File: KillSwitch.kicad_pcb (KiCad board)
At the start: 2 copper layers, 64 x 31 mm, 28 parts, among them J0 Screw_Terminal_1x04, J3 CONN_01X02, Q0 IRF1324PBF, Q1 IRF1324PBF, Q2 IRF1324PBF, Q3 IRF1324PBF, U0 NC7SZ08, U1 TPS62175, U2 4013

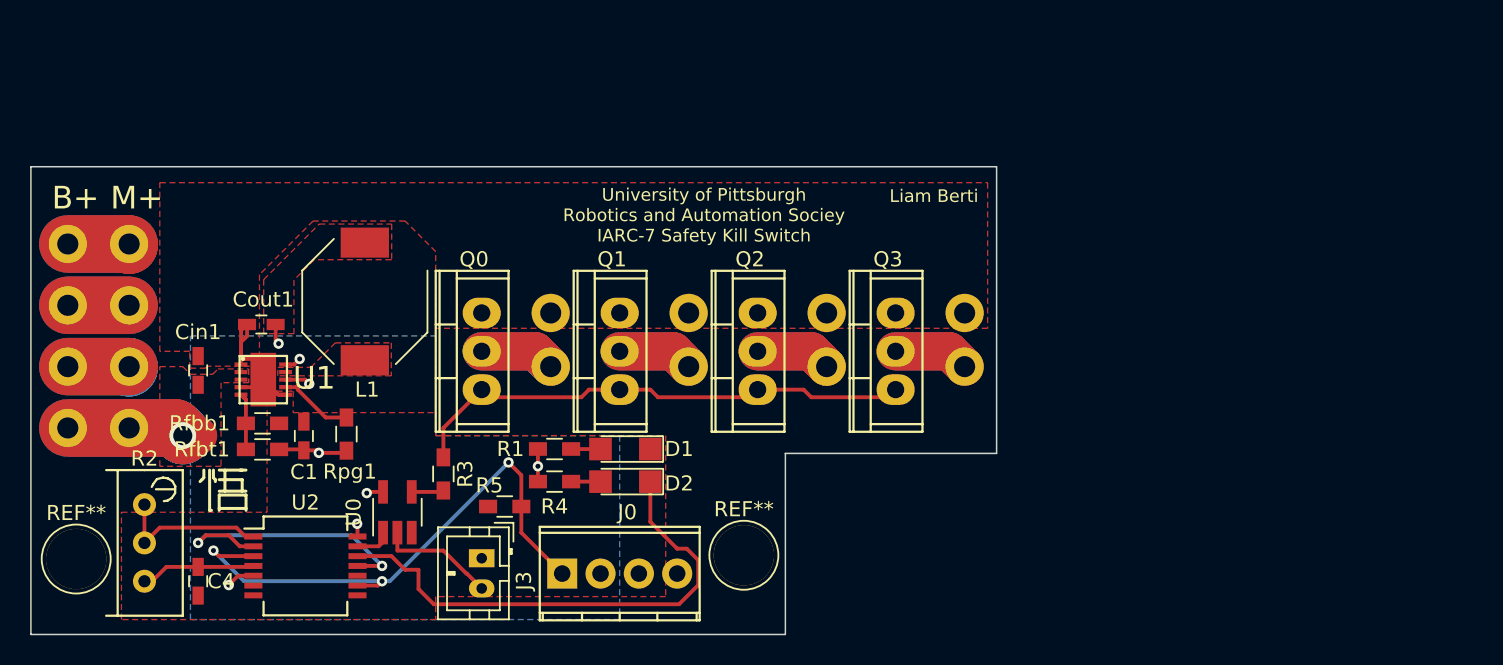
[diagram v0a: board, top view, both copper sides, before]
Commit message: new switch
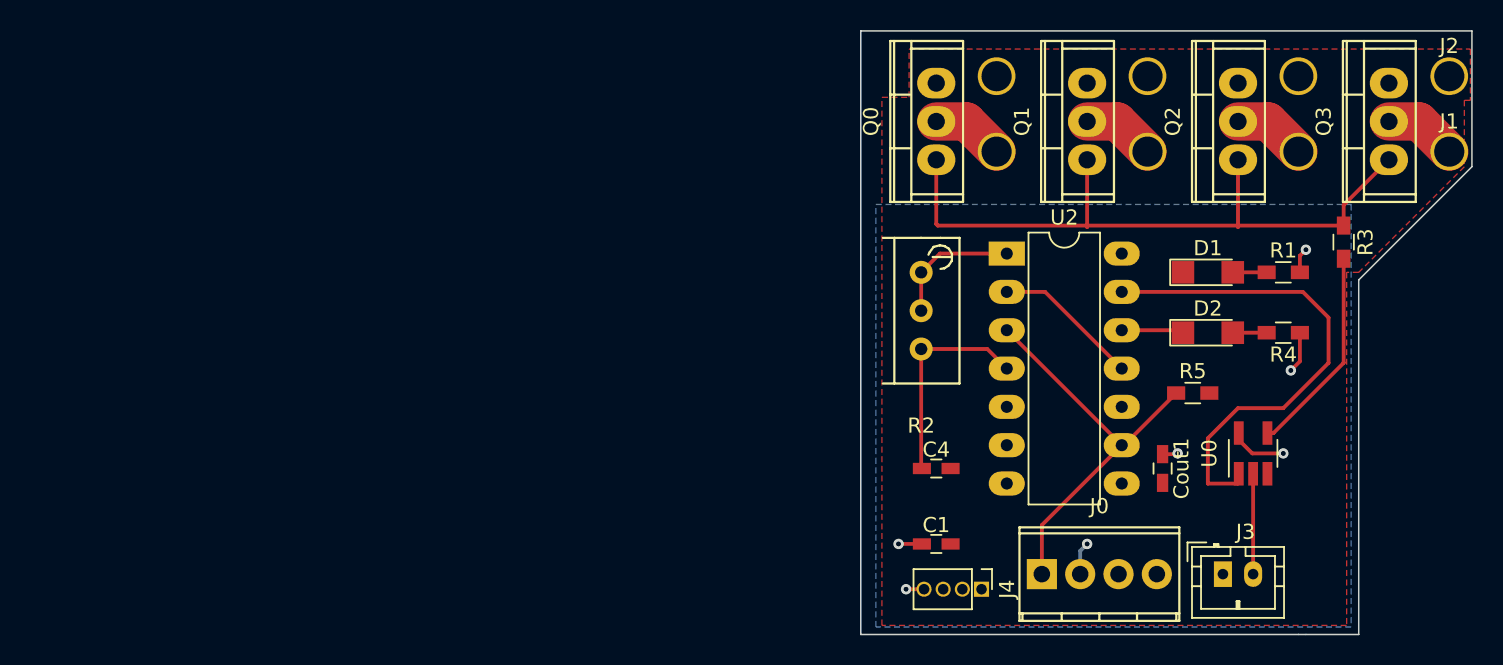
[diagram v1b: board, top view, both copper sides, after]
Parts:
- removed ? (x2): CONN_01X08, Wire_Pads:barrel_connector
- removed Cin1: 2.2uF, Capacitors_SMD:C_0603_HandSoldering
- removed L1: 10uH, 0.036Ohm, Inductors:Inductor_Bourns-SRU8043
- removed REF** (x2): 1pin, UserParts:4mmhole
- removed Rfbb1: 383k, Resistors_SMD:R_0603_HandSoldering
- removed Rfbt1: 2Meg, Resistors_SMD:R_0603_HandSoldering
- removed Rpg1: 100k, Resistors_SMD:R_0603_HandSoldering
- removed U1: TPS62175, Housings_SON:SON-10
- added J1: CONN_01X04, Wire_Pads:barrel_connector, F.Cu at (189.0, 56.0)
- added J2: CONN_01X04, Wire_Pads:barrel_connector, F.Cu at (218.0, 51.0)
- added J4: CONN_01X04, Socket_Strips:Socket_Strip_Straight_1x04_Pitch1.27mm, F.Cu at (184.0, 94.0)
- U2: footprint Housings_SSOP:SSOP-14_5.3x6.2mm_Pitch0.65mm -> Housings_DIP:DIP-14_W7.62mm_LongPads
- moved R3 61.6 mm to (208.0, 71.0)
- moved Cout1 60.5 mm to (196.0, 86.0), turned to 270 degrees
- moved U0 56.8 mm to (202.0, 85.0)
- moved R2 53.7 mm to (180.0, 73.0)
- moved U2 50.9 mm to (185.7, 71.8)
- moved R1 49.7 mm to (204.0, 73.0), turned to 0 degrees
- moved C4 49.5 mm to (181.0, 86.0), turned to 0 degrees
- moved R4 49.3 mm to (204.0, 77.0), turned to 180 degrees
- moved J3 49.1 mm to (200.0, 93.0), turned to 0 degrees
- moved R5 46.2 mm to (198.0, 81.0), turned to 0 degrees
- moved C1 42.5 mm to (181.0, 91.0), turned to 0 degrees
- moved D1 40.3 mm to (199.0, 73.0), turned to 0 degrees
- moved D2 39.8 mm to (199.0, 77.0), turned to 0 degrees
- moved Q3 36.1 mm to (211.0, 63.0)
- moved Q2 35.3 mm to (201.0, 63.0)
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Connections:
- J0 pad 4: Net-(J0-Pad4) -> (no net)
- U2 pad 7: VSS -> Earth
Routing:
- net /AND1: track 2.41 -> 33.1 mm
- net Net-(D2-Pad1): track 33.7 -> 4.36 mm
- net /VbattPos: track 18.1 -> 0.00 mm, vias 2 -> 0
- net Earth: track 13.6 -> 0.00 mm
- net Net-(J1-Pad8): track 12.4 -> 0.00 mm
- net Net-(J1-Pad6): track 12.3 -> 0.00 mm
- net /GATE: track 34.2 -> 46.0 mm
- net Net-(R3-Pad2): track 2.14 -> 13.9 mm
- net /PWM: track 37.0 -> 26.6 mm, vias 3 -> 0
- net Net-(U2-Pad11): track 19.0 -> 9.72 mm, vias 2 -> 0
- net Net-(J1-Pad7): track 8.13 -> 0.00 mm
- net Net-(J2-Pad4): track 11.4 -> 4.83 mm
- net Net-(J2-Pad2): track 11.4 -> 4.83 mm
- net Net-(C4-Pad1): track 7.73 -> 14.2 mm
- net Net-(J2-Pad1): track 9.99 -> 4.83 mm
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- removed copper zone on F.Cu, net +5V
- removed copper zone on F.Cu, net /VbattPos
- removed copper zone on F.Cu, net Net-(L1-Pad2)
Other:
- board size 64 x 31 mm -> 40.5 x 40 mm
- board text removed: "B+"
- board text removed: "Liam Berti"
- board text removed: "M+"
- board text removed: "University of Pittsburgh Robotics and Automation Sociey IARC-7 Safety Kill Switch"
